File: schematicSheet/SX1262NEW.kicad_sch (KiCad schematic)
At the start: 38 parts, among them U1 SX1262IMLTRT, U2 PE4259-63, Y1 32 MHz TCXO

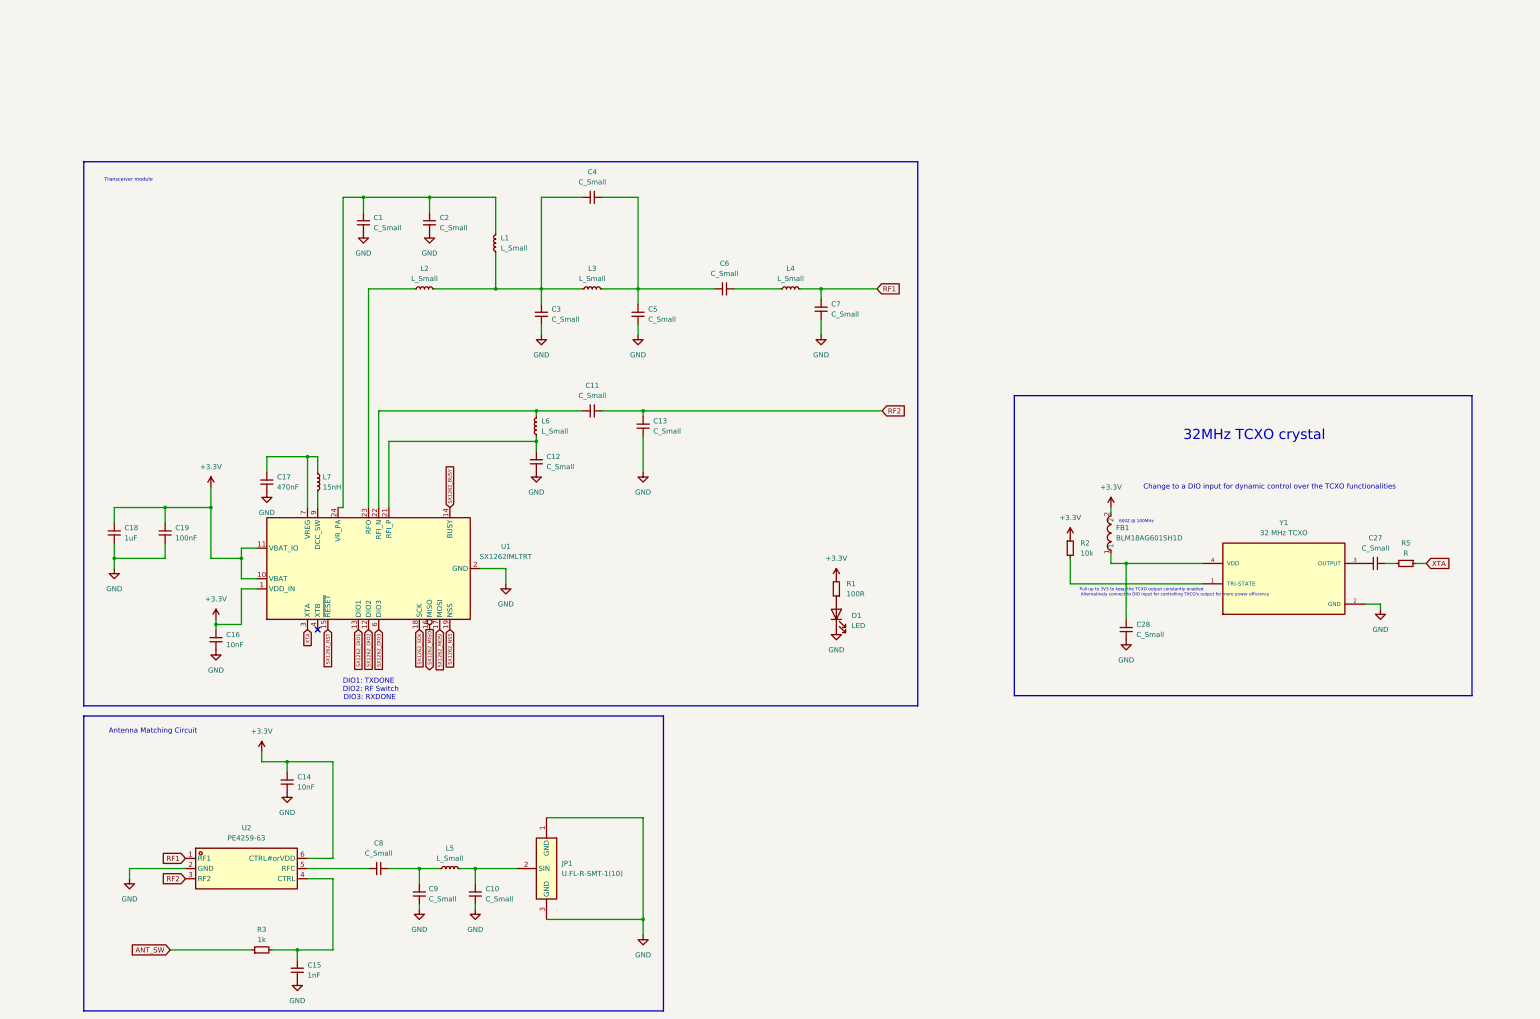
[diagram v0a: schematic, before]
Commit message: update
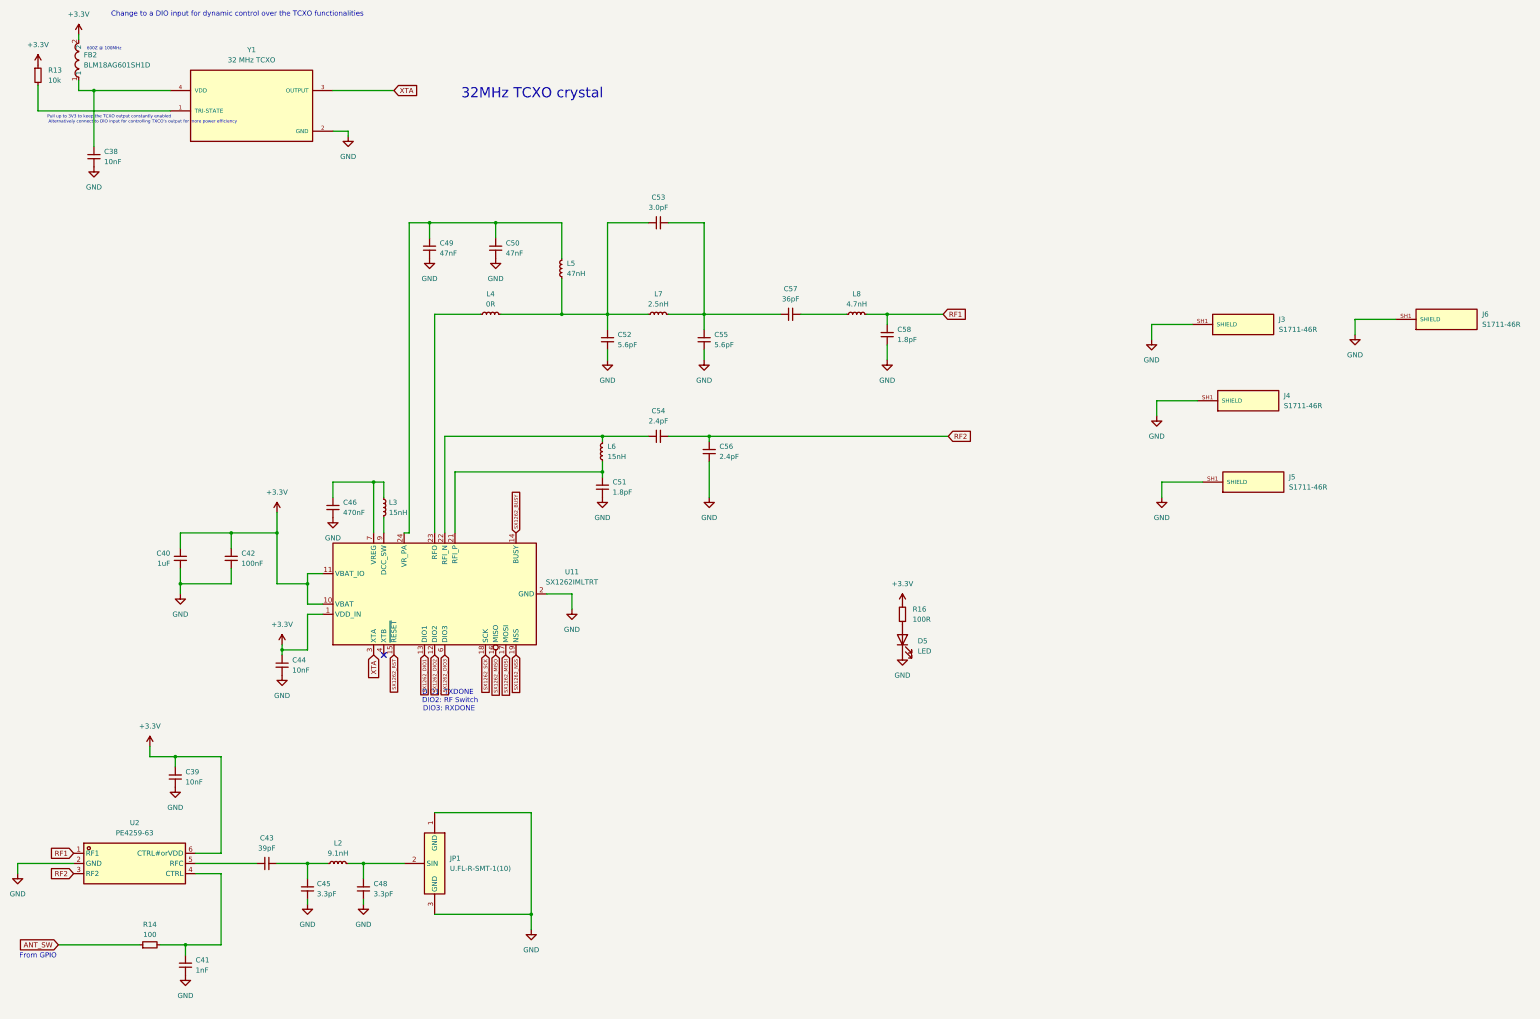
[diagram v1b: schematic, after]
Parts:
- removed C1, C10, C11, C12, C13, C2, C3, C4, C5, C6, C7, C8, C9: C_Small, Capacitor_SMD:C_0201_0603Metric, symbol Device:C_Small
- removed C14, C16: 10nF, Capacitor_SMD:C_0201_0603Metric, symbol Device:C_Small
- removed C15: 1nF, Capacitor_SMD:C_0201_0603Metric, symbol Device:C_Small
- removed C17: 470nF, Capacitor_SMD:C_0201_0603Metric, symbol Device:C_Small
- removed C18: 1uF, Capacitor_SMD:C_0402_1005Metric, symbol Device:C_Small
- removed C19: 100nF, Capacitor_SMD:C_0201_0603Metric, symbol Device:C_Small
- removed C27, C28: C_Small, Capacitor_SMD:C_0402_1005Metric, symbol Device:C_Small
- removed D1: LED, LED_SMD:LED_0402_1005Metric, symbol Device:LED
- removed FB1: BLM18AG601SH1D, EasyEDA:L0603, symbol EasyEDA:BLM18AG601SH1D
- removed L1: L_Small, Inductor_SMD:L_0201_0603Metric, symbol Device:L_Small
- removed R1: 100R, Resistor_SMD:R_0201_0603Metric, symbol Device:R_Small
- removed R2: 10k, Resistor_SMD:R_0402_1005Metric, symbol Device:R_Small
- removed R3: 1k, Resistor_SMD:R_0402_1005Metric, symbol Device:R_Small
- removed R5: R, Resistor_SMD:R_0402_1005Metric, symbol Device:R_Small
- removed U1: SX1262IMLTRT, Package_DFN_QFN:QFN-24-1EP_4x4mm_P0.5mm_EP2.6x2.6mm, symbol RF:SX1262IMLTRT
- added C38: 10nF, Capacitor_SMD:C_0402_1005Metric, symbol Device:C_Small
- added C39, C44: 10nF, Capacitor_SMD:C_0201_0603Metric, symbol Device:C_Small
- added C40: 1uF, Capacitor_SMD:C_0402_1005Metric, symbol Device:C_Small
- added C41: 1nF, Capacitor_SMD:C_0201_0603Metric, symbol Device:C_Small
- added C42: 100nF, Capacitor_SMD:C_0201_0603Metric, symbol Device:C_Small
- added C43: 39pF, Capacitor_SMD:C_0201_0603Metric, symbol Device:C_Small
- added C45, C48: 3.3pF, Capacitor_SMD:C_0201_0603Metric, symbol Device:C_Small
- added C46: 470nF, Capacitor_SMD:C_0201_0603Metric, symbol Device:C_Small
- added C49, C50: 47nF, Capacitor_SMD:C_0201_0603Metric, symbol Device:C_Small
- added C51, C58: 1.8pF, Capacitor_SMD:C_0201_0603Metric, symbol Device:C_Small
- added C52, C55: 5.6pF, Capacitor_SMD:C_0201_0603Metric, symbol Device:C_Small
- added C53: 3.0pF, Capacitor_SMD:C_0201_0603Metric, symbol Device:C_Small
- added C54, C56: 2.4pF, Capacitor_SMD:C_0201_0603Metric, symbol Device:C_Small
- added C57: 36pF, Capacitor_SMD:C_0201_0603Metric, symbol Device:C_Small
- added D5: LED, LED_SMD:LED_0402_1005Metric, symbol Device:LED
- added FB2: BLM18AG601SH1D, EasyEDA:L0603, symbol EasyEDA:BLM18AG601SH1D
- added J3, J4, J5, J6: S1711-46R, shield:HARWIN_S1711-46R, symbol S1711-46R:S1711-46R
- added L8: 4.7nH, Inductor_SMD:L_0201_0603Metric, symbol Device:L_Small
- added R13: 10k, Resistor_SMD:R_0402_1005Metric, symbol Device:R_Small
- added R14: 100, Resistor_SMD:R_0402_1005Metric, symbol Device:R_Small
- added R16: 100R, Resistor_SMD:R_0201_0603Metric, symbol Device:R_Small
- added U11: SX1262IMLTRT, Package_DFN_QFN:QFN-24-1EP_4x4mm_P0.5mm_EP2.6x2.6mm, symbol RF:SX1262IMLTRT
- L2: value L_Small -> 9.1nH
- L3: value L_Small -> 15nH; footprint Inductor_SMD:L_0201_0603Metric -> Inductor_SMD:L_0402_1005Metric
- L4: value L_Small -> 0R
- L5: value L_Small -> 47nH
- L6: value L_Small -> 15nH
- L7: value 15nH -> 2.5nH; footprint Inductor_SMD:L_0402_1005Metric -> Inductor_SMD:L_0201_0603Metric
- Y1: footprint TCXO:OSC_ECS-TXO-2520-33-320-AN-TR -> TXTO:OSC_ECS-TXO-2520-33-320-AN-TR
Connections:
- net +3.3V: now also C39.2, C40.1, C42.1, C44.1, FB2.2, R13.1, R16.2, U11.1 (VDD_IN), U11.10 (VBAT), U11.11 (VBAT_IO)
- net ANT_SW: now also R14.1
- net GND: now also C38.2, C39.1, C40.2, C41.1, C42.2, C44.2, C45.1, C46.2, C48.1, C49.2, C50.2, C51.1, C52.2, C55.2, C56.1, C58.1, D5.1 (K), J3.SH1 (SHIELD), J4.SH1 (SHIELD), J5.SH1 (SHIELD), J6.SH1 (SHIELD), U11.2 (GND), U11.20 (GND), U11.25 (GND), U11.5 (GND), U11.8 (GND)
- net RF1: now also C58.2, L8.2; no longer L4.2
- net RF2: now also C54.2, C56.2
- net SX1262_BUSY: now also U11.14 (BUSY)
- net SX1262_DIO1: now also U11.13 (DIO1)
- net SX1262_DIO2: now also U11.12 (DIO2)
- net SX1262_DIO3: now also U11.6 (DIO3)
- net SX1262_MISO: now also U11.16 (MISO)
- net SX1262_MOSI: now also U11.17 (MOSI)
- net SX1262_NSS: now also U11.19 (NSS)
- net SX1262_RST: now also U11.15 (~{RESET})
- net SX1262_SCK: now also U11.18 (SCK)
- net XTA: now also Y1.3 (OUTPUT), U11.3 (XTA)
- net at L2.2: now also JP1.2 (SIN), C48.2; no longer L3.1
- net at L3.2: now also U11.9 (DCC_SW)
- net at L5.1: now also L4.2, L7.1, C52.1, C53.1
- net at U2.5 (RFC): now also C43.2
- net at L6.1: now also C51.2, U11.21 (RFI_P)
- net at L6.2: now also C54.1, U11.22 (RFI_N)
- net at L4.1: now also U11.23 (RFO)
- net at Y1.4 (VDD): now also C38.1, FB2.1
- net at L2.1: now also C43.1, C45.2
- net at L7.2: now also C53.2, C55.1, C57.1
- net at U2.4 (CTRL): now also C41.2, R14.2
- net at L5.2: now also C49.1, C50.1, U11.24 (VR_PA); no longer JP1.2 (SIN)
- net at Y1.1 (TRI-STATE): now also R13.2
- new net: C57.2, L8.1
- new net: C46.1, L3.1, U11.7 (VREG)
- new net: D5.2 (A), R16.1
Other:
- note added: "From GPIO"
- note removed: "Antenna Matching Circuit"
- note removed: "Transceiver module"
